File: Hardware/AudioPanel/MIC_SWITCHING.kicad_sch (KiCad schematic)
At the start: 22 parts, among them U119 ADG729, U120 ADG729, U122 MCP6004, U123 ADS7830, U124 MCP6004, U125 MCP47FVB08, U126 MCP47FVB08

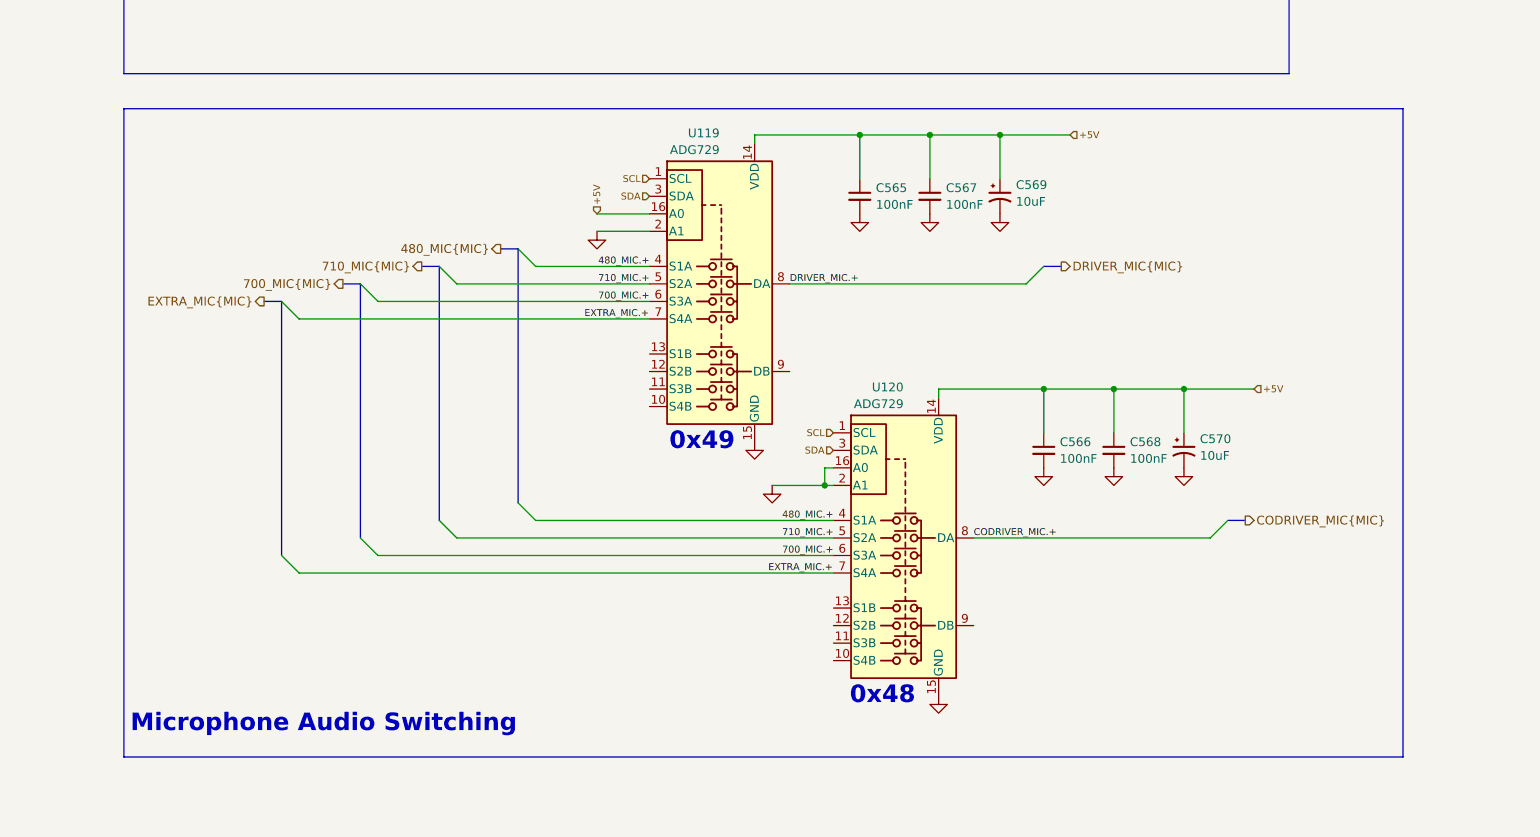
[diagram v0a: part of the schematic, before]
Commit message: Cleaned up stuff, defined more busses
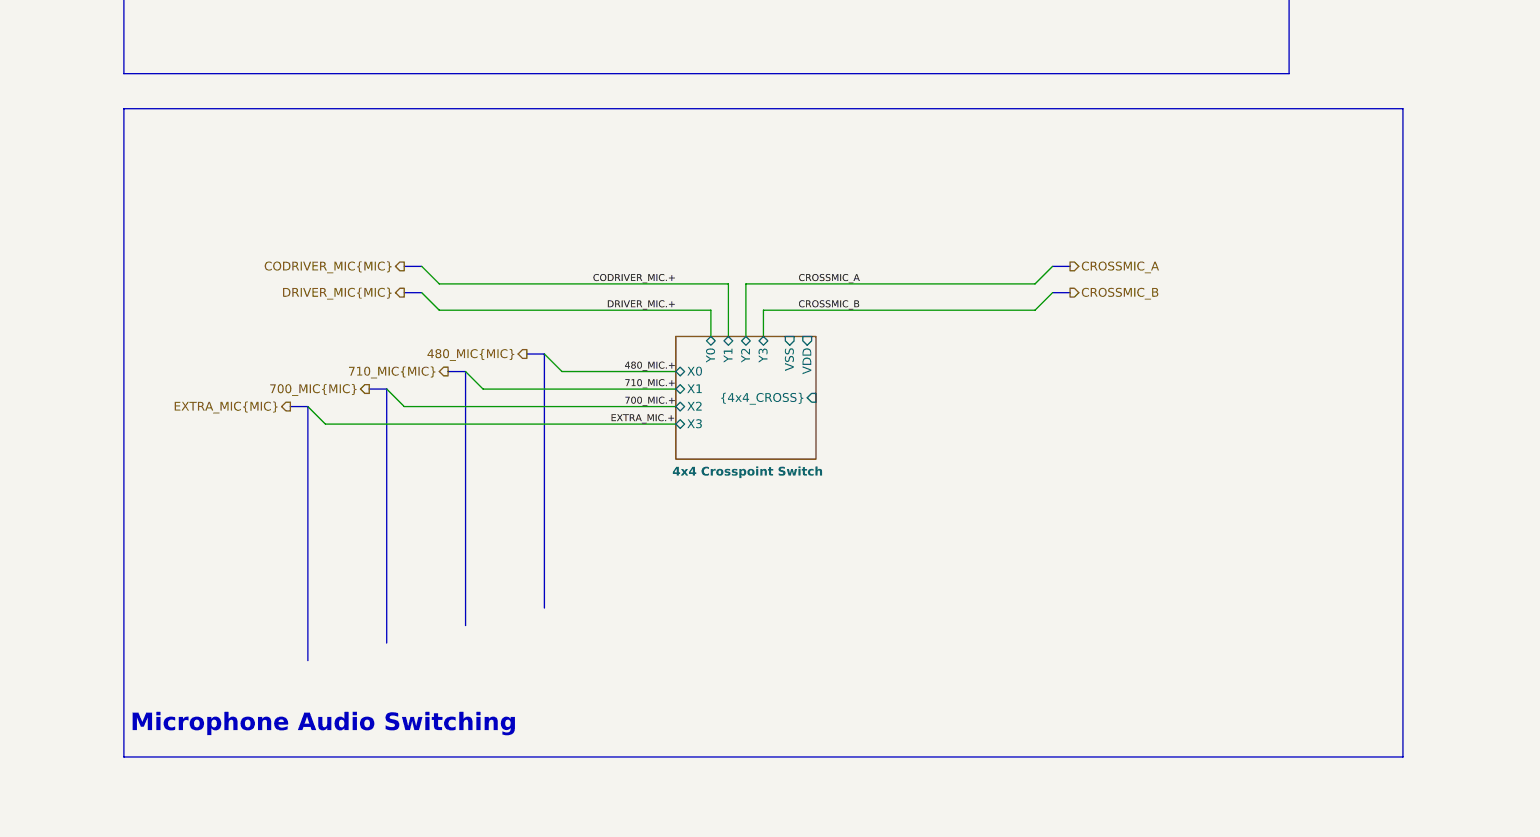
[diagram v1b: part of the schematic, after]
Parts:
- removed C565, C566, C567, C568: 100nF, symbol Device:C_Small
- removed C569, C570: 10uF, symbol Device:C_Polarized_Small_US
- removed U119, U120: ADG729, Package_SO:TSSOP-16_4.4x5mm_P0.65mm, symbol Analog_Switch:ADG729
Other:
- added sheet 4x4 Crosspoint Switch (Crosspoint_4x4_4066.kicad_sch)
- note removed: "0x48"
- note removed: "0x49"
